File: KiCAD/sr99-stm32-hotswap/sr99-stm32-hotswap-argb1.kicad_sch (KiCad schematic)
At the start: 36 parts, among them U10 IS31FL3743B, U11 AP2112K, U12 AP2112K, U9 IS31FL3743B

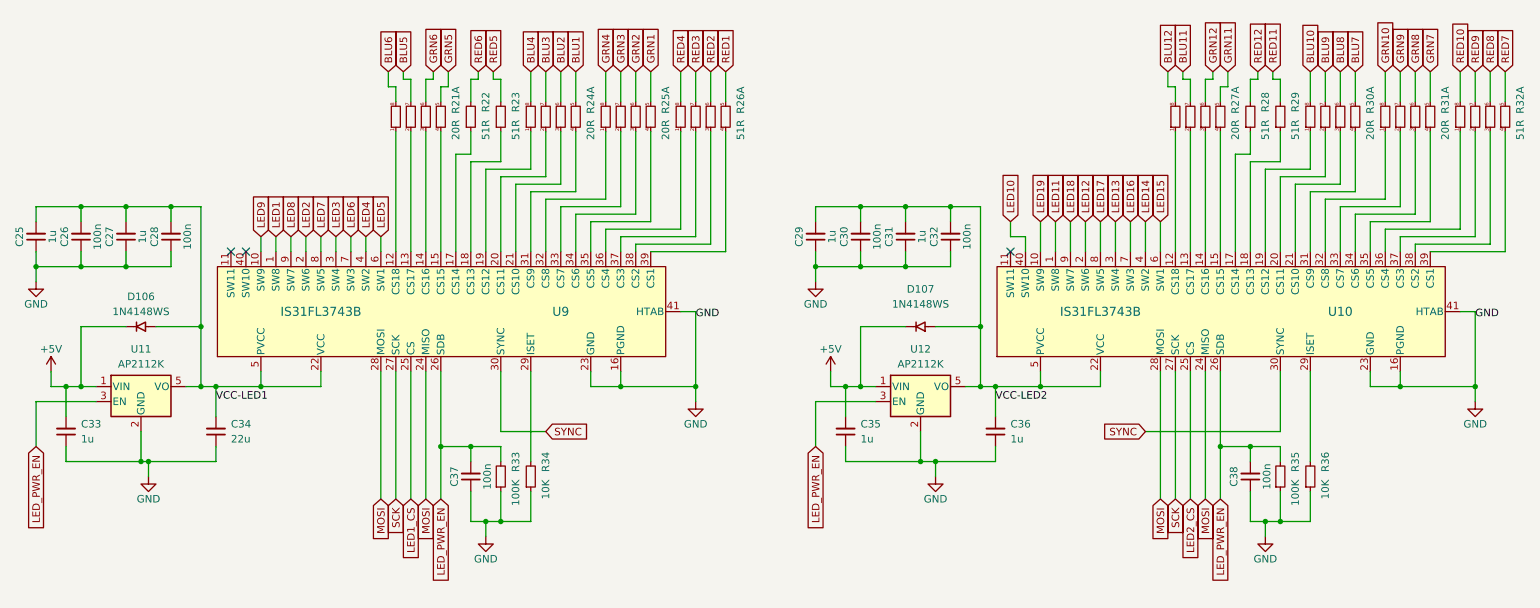
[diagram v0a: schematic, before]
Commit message: wip-2025-11-23
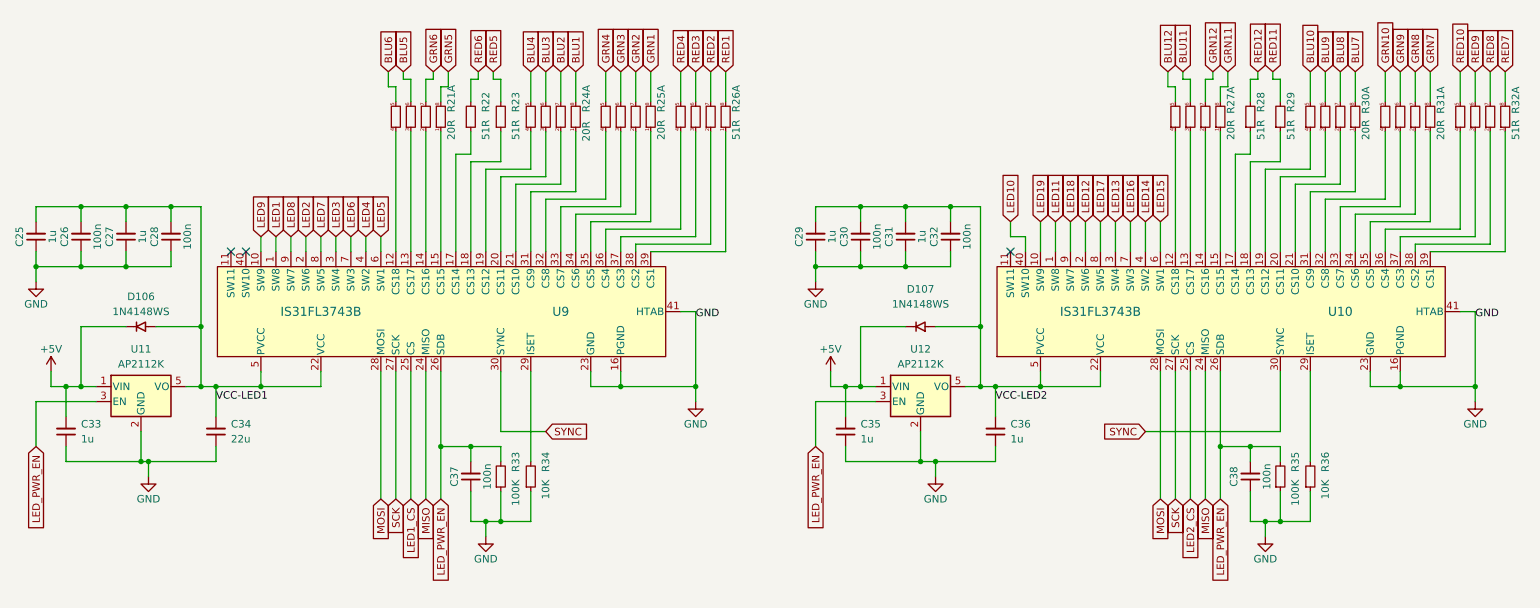
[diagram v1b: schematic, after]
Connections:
- net BLU1: now also R24.8; no longer R24.5
- net BLU10: now also R30.5; no longer R30.8
- net BLU11: now also R27.6; no longer R27.7
- net BLU12: now also R27.5; no longer R27.8
- net BLU2: now also R24.7; no longer R24.6
- net BLU3: now also R24.6; no longer R24.7
- net BLU4: now also R24.5; no longer R24.8
- net BLU5: now also R21.6; no longer R21.7
- net BLU6: now also R21.5; no longer R21.8
- net BLU7: now also R30.8; no longer R30.5
- net BLU8: now also R30.7; no longer R30.6
- net BLU9: now also R30.6; no longer R30.7
- net GRN1: now also R25.8; no longer R25.5
- net GRN10: now also R31.5; no longer R31.8
- net GRN11: now also R27.8; no longer R27.5
- net GRN12: now also R27.7; no longer R27.6
- net GRN2: now also R25.7; no longer R25.6
- net GRN3: now also R25.6; no longer R25.7
- net GRN4: now also R25.5; no longer R25.8
- net GRN5: now also R21.8; no longer R21.5
- net GRN6: now also R21.7; no longer R21.6
- net GRN7: now also R31.8; no longer R31.5
- net GRN8: now also R31.7; no longer R31.6
- net GRN9: now also R31.6; no longer R31.7
- net MOSI: no longer U10.24 (MISO), U9.24 (MISO)
- net RED1: now also R26.8; no longer R26.5
- net RED10: now also R32.5; no longer R32.8
- net RED2: now also R26.7; no longer R26.6
- net RED3: now also R26.6; no longer R26.7
- net RED4: now also R26.5; no longer R26.8
- net RED7: now also R32.8; no longer R32.5
- net RED8: now also R32.7; no longer R32.6
- net RED9: now also R32.6; no longer R32.7
- net at R32.1: now also U10.39 (CS1); no longer U10.36 (CS4)
- net at R31.1: now also U10.35 (CS5); no longer U10.32 (CS8)
- net at R26.4: now also U9.36 (CS4); no longer U9.39 (CS1)
- net at R32.4: now also U10.36 (CS4); no longer U10.39 (CS1)
- net at R31.4: now also U10.32 (CS8); no longer U10.35 (CS5)
- net at R27.3: now also U10.13 (CS17); no longer U10.14 (CS16)
- net at R21.1: now also U9.15 (CS15); no longer U9.12 (CS18)
- net at R30.1: now also U10.31 (CS9); no longer U10.19 (CS12)
- net at U9.13 (CS17): now also R21.3; no longer R21.2
- net at U9.14 (CS16): now also R21.2; no longer R21.3
- net at R21.4: now also U9.12 (CS18); no longer U9.15 (CS15)
- net at U9.19 (CS12): now also R24.4; no longer R24.1
- net at U9.20 (CS11): now also R24.3; no longer R24.2
- net at U9.21 (CS10): now also R24.2; no longer R24.3
- net at U9.31 (CS9): now also R24.1; no longer R24.4
- net at U9.32 (CS8): now also R25.4; no longer R25.1
- net at U9.33 (CS7): now also R25.3; no longer R25.2
- net at U9.34 (CS6): now also R25.2; no longer R25.3
- net at U9.35 (CS5): now also R25.1; no longer R25.4
- net at R26.1: now also U9.39 (CS1); no longer U9.36 (CS4)
- net at U9.37 (CS3): now also R26.3; no longer R26.2
- net at U9.38 (CS2): now also R26.2; no longer R26.3
- net at R32.3: now also U10.37 (CS3); no longer U10.38 (CS2)
- net at R27.4: now also U10.12 (CS18); no longer U10.15 (CS15)
- net at R31.2: now also U10.34 (CS6); no longer U10.33 (CS7)
- net at R32.2: now also U10.38 (CS2); no longer U10.37 (CS3)
- net at R30.3: now also U10.20 (CS11); no longer U10.21 (CS10)
- net at R27.1: now also U10.15 (CS15); no longer U10.12 (CS18)
- net at R30.4: now also U10.19 (CS12); no longer U10.31 (CS9)
- net at R27.2: now also U10.14 (CS16); no longer U10.13 (CS17)
- net at R30.2: now also U10.21 (CS10); no longer U10.20 (CS11)
- net at R31.3: now also U10.33 (CS7); no longer U10.34 (CS6)
- new net MISO: U10.24 (MISO), U9.24 (MISO)
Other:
- moved on the sheet: R21A, R24A, R25A, R26A, R27A, R30A, R31A, R32A

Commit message: wip
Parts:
- C25, C26, C27, C28, C29, C30, C31, C32, C37, C38: footprint Capacitor_SMD:C_0603_1608Metric_Pad1.08x0.95mm_HandSolder -> Capacitor_SMD:C_0402_1005Metric
- C33, C34, C35, C36: footprint Capacitor_SMD:C_0603_1608Metric -> Capacitor_SMD:C_0402_1005Metric
- R22, R23, R28, R29, R33, R34, R35, R36: footprint Resistor_SMD:R_0603_1608Metric -> Resistor_SMD:R_0402_1005Metric
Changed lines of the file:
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@@
 			)
 		)
-		(property "Footprint" "Resistor_SMD:R_0603_1608Metric"
+		(property "Footprint" "Resistor_SMD:R_0402_1005Metric"
 			(at 241.3 114.3 0)
 			(effects
@@
 			)
 		)
-		(property "Footprint" "Capacitor_SMD:C_0603_1608Metric_Pad1.08x0.95mm_HandSolder"
+		(property "Footprint" "Capacitor_SMD:C_0402_1005Metric"
 			(at 48.26 73.66 0)
 			(effects
@@
 			)
 		)
-		(property "Footprint" "Resistor_SMD:R_0603_1608Metric"
+		(property "Footprint" "Resistor_SMD:R_0402_1005Metric"
 			(at 236.22 53.34 0)
 			(effects
@@
 			)
 		)
-		(property "Footprint" "Resistor_SMD:R_0603_1608Metric"
+		(property "Footprint" "Resistor_SMD:R_0402_1005Metric"
 			(at 109.22 114.3 0)
 			(effects
@@
 			)
 		)
-		(property "Footprint" "Capacitor_SMD:C_0603_1608Metric_Pad1.08x0.95mm_HandSolder"
+		(property "Footprint" "Capacitor_SMD:C_0402_1005Metric"
 			(at 172.72 73.66 0)
 			(effects
@@
 			)
 		)
-		(property "Footprint" "Capacitor_SMD:C_0603_1608Metric"
+		(property "Footprint" "Capacitor_SMD:C_0402_1005Metric"
 			(at 194.31 106.934 0)
 			(effects
@@
 			)
 		)
-		(property "Footprint" "Capacitor_SMD:C_0603_1608Metric_Pad1.08x0.95mm_HandSolder"
+		(property "Footprint" "Capacitor_SMD:C_0402_1005Metric"
 			(at 33.02 73.66 0)
 			(effects
@@
 			)
 		)
-		(property "Footprint" "Capacitor_SMD:C_0603_1608Metric_Pad1.08x0.95mm_HandSolder"
+		(property "Footprint" "Capacitor_SMD:C_0402_1005Metric"
 			(at 180.34 73.66 0)
 			(effects
@@
 			)
 		)
-		(property "Footprint" "Capacitor_SMD:C_0603_1608Metric_Pad1.08x0.95mm_HandSolder"
+		(property "Footprint" "Capacitor_SMD:C_0402_1005Metric"
 			(at 165.1 73.66 0)
 			(effects
@@
 			)
 		)
-		(property "Footprint" "Capacitor_SMD:C_0603_1608Metric"
+		(property "Footprint" "Capacitor_SMD:C_0402_1005Metric"
 			(at 36.83 106.934 0)
 			(effects
@@
 			)
 		)
-		(property "Footprint" "Resistor_SMD:R_0603_1608Metric"
+		(property "Footprint" "Resistor_SMD:R_0402_1005Metric"
 			(at 104.14 53.34 0)
 			(effects
@@
 			)
 		)
-		(property "Footprint" "Capacitor_SMD:C_0603_1608Metric_Pad1.08x0.95mm_HandSolder"
+		(property "Footprint" "Capacitor_SMD:C_0402_1005Metric"
 			(at 99.06 114.3 0)
 			(effects
@@
 			)
 		)
-		(property "Footprint" "Resistor_SMD:R_0603_1608Metric"
+		(property "Footprint" "Resistor_SMD:R_0402_1005Metric"
 			(at 104.14 114.3 0)
 			(effects
@@
 			)
 		)
-		(property "Footprint" "Capacitor_SMD:C_0603_1608Metric"
+		(property "Footprint" "Capacitor_SMD:C_0402_1005Metric"
 			(at 62.23 106.934 0)
 			(effects
@@
 			)
 		)
-		(property "Footprint" "Resistor_SMD:R_0603_1608Metric"
+		(property "Footprint" "Resistor_SMD:R_0402_1005Metric"
 			(at 236.22 114.3 0)
 			(effects
@@
 			)
 		)
-		(property "Footprint" "Resistor_SMD:R_0603_1608Metric"
+		(property "Footprint" "Resistor_SMD:R_0402_1005Metric"
 			(at 99.06 53.34 0)
 			(effects
@@
 			)
 		)
-		(property "Footprint" "Resistor_SMD:R_0603_1608Metric"
+		(property "Footprint" "Resistor_SMD:R_0402_1005Metric"
 			(at 231.14 53.34 0)
 			(effects
@@
 			)
 		)
-		(property "Footprint" "Capacitor_SMD:C_0603_1608Metric_Pad1.08x0.95mm_HandSolder"
+		(property "Footprint" "Capacitor_SMD:C_0402_1005Metric"
 			(at 157.48 73.66 0)
 			(effects
@@
 			)
 		)
-		(property "Footprint" "Capacitor_SMD:C_0603_1608Metric_Pad1.08x0.95mm_HandSolder"
+		(property "Footprint" "Capacitor_SMD:C_0402_1005Metric"
 			(at 40.64 73.66 0)
 			(effects
@@
 			)
 		)
-		(property "Footprint" "Capacitor_SMD:C_0603_1608Metric"
+		(property "Footprint" "Capacitor_SMD:C_0402_1005Metric"
 			(at 168.91 106.934 0)
 			(effects
@@
 			)
 		)
-		(property "Footprint" "Capacitor_SMD:C_0603_1608Metric_Pad1.08x0.95mm_HandSolder"
+		(property "Footprint" "Capacitor_SMD:C_0402_1005Metric"
 			(at 25.4 73.66 0)
 			(effects
@@
 			)
 		)
-		(property "Footprint" "Capacitor_SMD:C_0603_1608Metric_Pad1.08x0.95mm_HandSolder"
+		(property "Footprint" "Capacitor_SMD:C_0402_1005Metric"
 			(at 231.14 114.3 0)
 			(effects
